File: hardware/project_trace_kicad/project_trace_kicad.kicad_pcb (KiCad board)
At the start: 4 copper layers, 100 x 100 mm, 97 parts, among them J204 Screw_Terminal_01x04, J205 Conn_Coaxial, J503 Screw_Terminal_01x04, U201 TLE2426xLP, U202 AQW280SX, U203 AQW282SX, U204 OPA2837IRUNT, U205 TS5A23159DGS, U206 OPA2837IRUNT, U301 THS4131IDR, U303 ADS1602, U304 MCP6499T, U305 LM4040DBZ-2.5, U306 LM4040DBZ-4.1, U501 UA78M33QDCYRQ1, U502 UA78M05QDCYRQ1

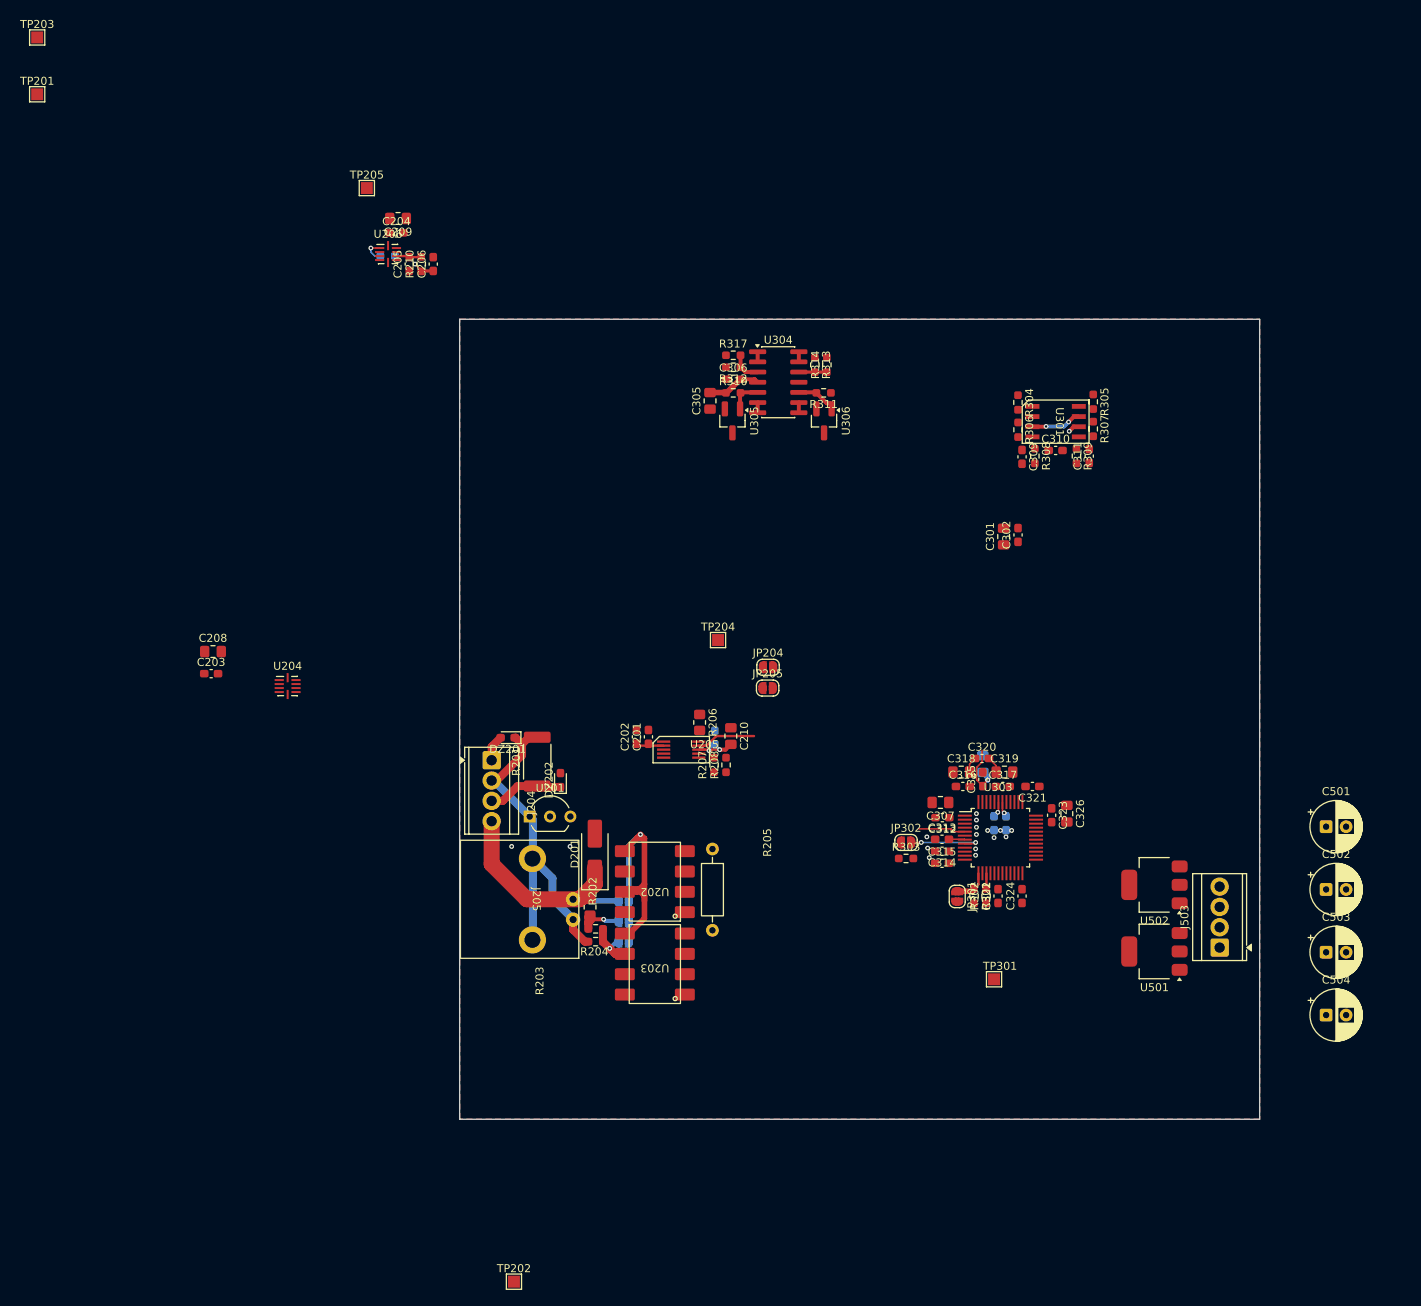
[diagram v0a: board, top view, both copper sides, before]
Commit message: Layout Broad Strokes, Fix STM32H7 Error
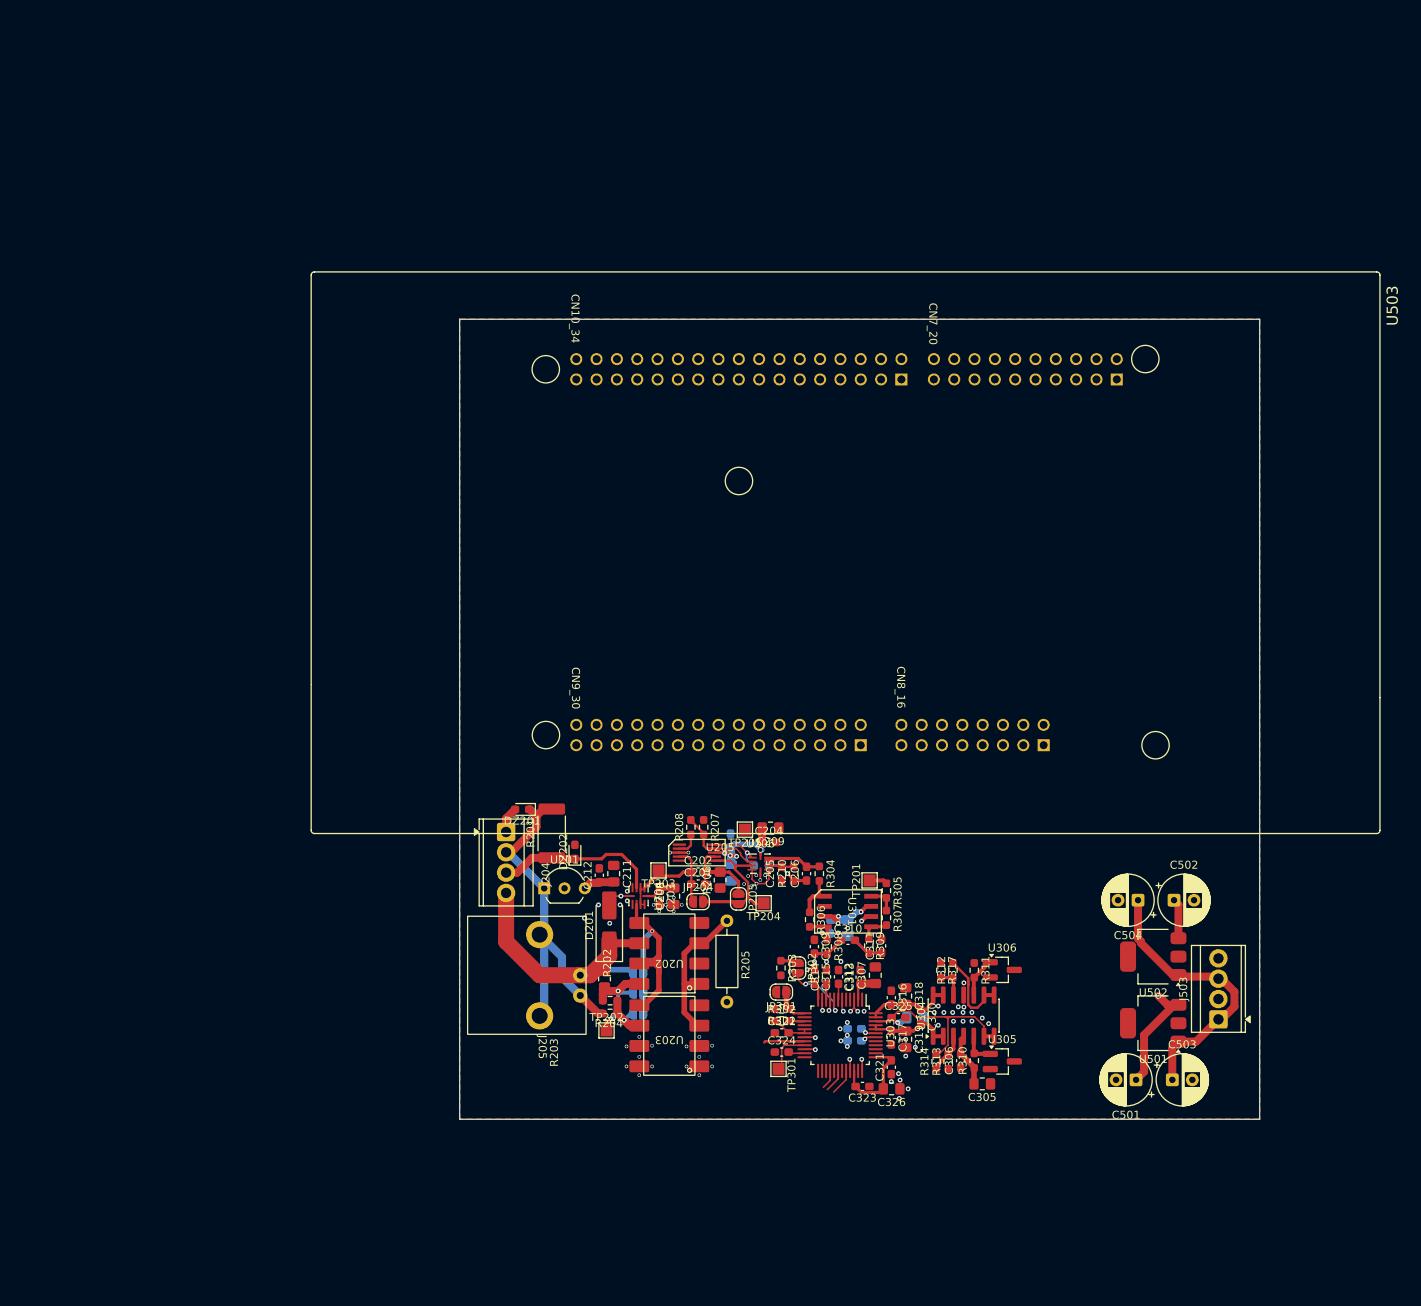
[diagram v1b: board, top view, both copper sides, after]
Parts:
- added C211: 10u, Capacitor_SMD:C_0805_2012Metric_Pad1.18x1.45mm_HandSolder, F.Cu at (119.3, 119.3)
- added C212: 100n, Capacitor_SMD:C_0603_1608Metric_Pad1.08x0.95mm_HandSolder, F.Cu at (117.5, 119.5)
- added U503: NUCLEO-H753ZI, ProjectTraceFootprints:MODULE_NUCLEO-H753ZI, F.Cu at (148.2, 79.1)
- C210, C301, C302: moved to B.Cu
- moved TP201 143.1 mm to (151.2, 120.1), turned to 90 degrees
- moved TP203 129.9 mm to (124.9, 118.9), turned to 180 degrees
- moved TP205 93.1 mm to (135.7, 113.8), turned to 180 degrees
- moved C305 91.9 mm to (165.3, 145.6), turned to 180 degrees
- moved C306 89.8 mm to (162.6, 142.7), turned to 90 degrees
- moved R209 89.4 mm to (137.7, 118.3)
- moved C206 89.4 mm to (143.4, 119.3)
- moved C204 89.3 mm to (138.7, 115.4)
- moved C209 89.3 mm to (138.9, 113.6)
- moved U206 89.3 mm to (137.6, 118.0)
- moved C205 89.3 mm to (140.3, 119.3)
- moved R210 89.3 mm to (141.8, 119.3)
- moved R310 88.7 mm to (164.3, 142.7), turned to 90 degrees
- moved R313 88.7 mm to (161.1, 142.8), turned to 90 degrees
- moved R314 88.2 mm to (159.6, 142.8)
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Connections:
- R206 pad 2: Net-(JP204-B) -> Net-(JP205-A)
- R312 pad 1: Net-(U304A-+) -> Net-(U304D-+)
- R313 pad 2: Net-(U304D-+) -> Net-(U304A-+)
- R314 pad 1: Net-(U304D-+) -> Net-(U304A-+)
- R317 pad 2: Net-(U304A-+) -> Net-(U304D-+)
- U205 pad 1: /Inputs/ACCouple.EN -> /Inputs/20dBGain.EN
- U205 pad 10: Net-(JP204-B) -> Net-(R209-Pad1)
- U205 pad 2: /Inputs/AttenBuffer -> Net-(R208-Pad1)
- U205 pad 4: Net-(R208-Pad1) -> /Inputs/AttenBuffer
- U205 pad 5: /Inputs/20dBGain.EN -> /Inputs/ACCouple.EN
- U205 pad 6: Net-(R209-Pad1) -> Net-(JP204-B)
- U205 pad 7: Net-(U206A--) -> Net-(JP205-A)
- U205 pad 9: Net-(JP205-A) -> Net-(U206A--)
- U304 pad 1: +4V -> +1V0
- U304 pad 13: +1V0 -> +4V
- U304 pad 14: +1V0 -> +4V
- U304 pad 2: +4V -> +1V0
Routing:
- net +3V3: track 0.00 -> 38.8 mm, vias 0 -> 2
- net Net-(J503-Pin_1): track 0.00 -> 35.5 mm
- net +5V: track 22.7 -> 55.6 mm, vias 5 -> 8
- net Net-(U202A-P1): track 0.00 -> 18.4 mm
- net GND: track 4.72 -> 22.4 mm, vias 17 -> 82
- net Net-(JP204-B): track 0.00 -> 17.6 mm
- net +2V5: track 8.56 -> 25.8 mm
- net /Inputs/AttenBuffer: track 3.50 -> 16.9 mm
- net Net-(U206A--): track 0.00 -> 11.0 mm
- net /Inputs/Ammeter.In: track 9.26 -> 20.2 mm
- net /Inputs/Attten.20dB: track 6.19 -> 16.2 mm, vias 1 -> 2
- net 4V1: track 1.27 -> 10.5 mm
- net /ADC/Signal.In: track 0.00 -> 8.42 mm
- net +4V: track 3.35 -> 11.1 mm
- net +1V0: track 3.57 -> 10.8 mm
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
